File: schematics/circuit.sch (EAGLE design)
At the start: 39 parts, among them IC2 TLC271D, U1 AD5241BRU1M-REEL7AD5241BRZ1M, X1 87758-1816

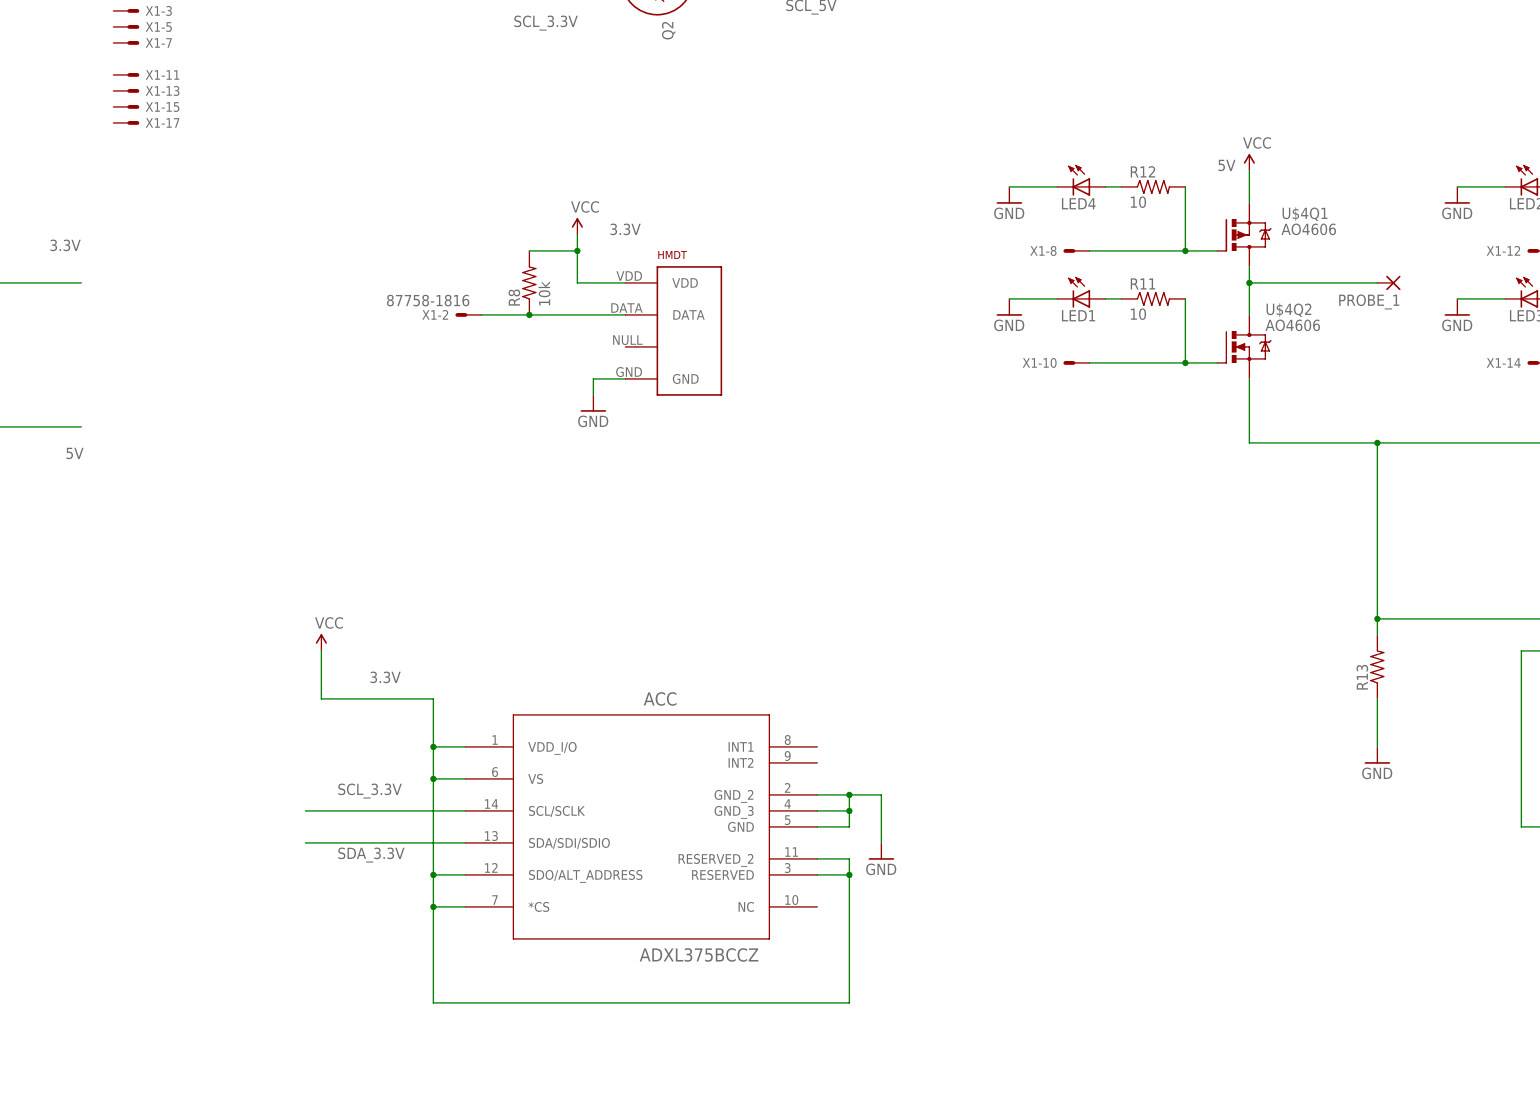
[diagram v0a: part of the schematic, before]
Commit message: почти закончили схему (кроме пережигателей, термисторов, выключателей и флешки) + начала разводить плату
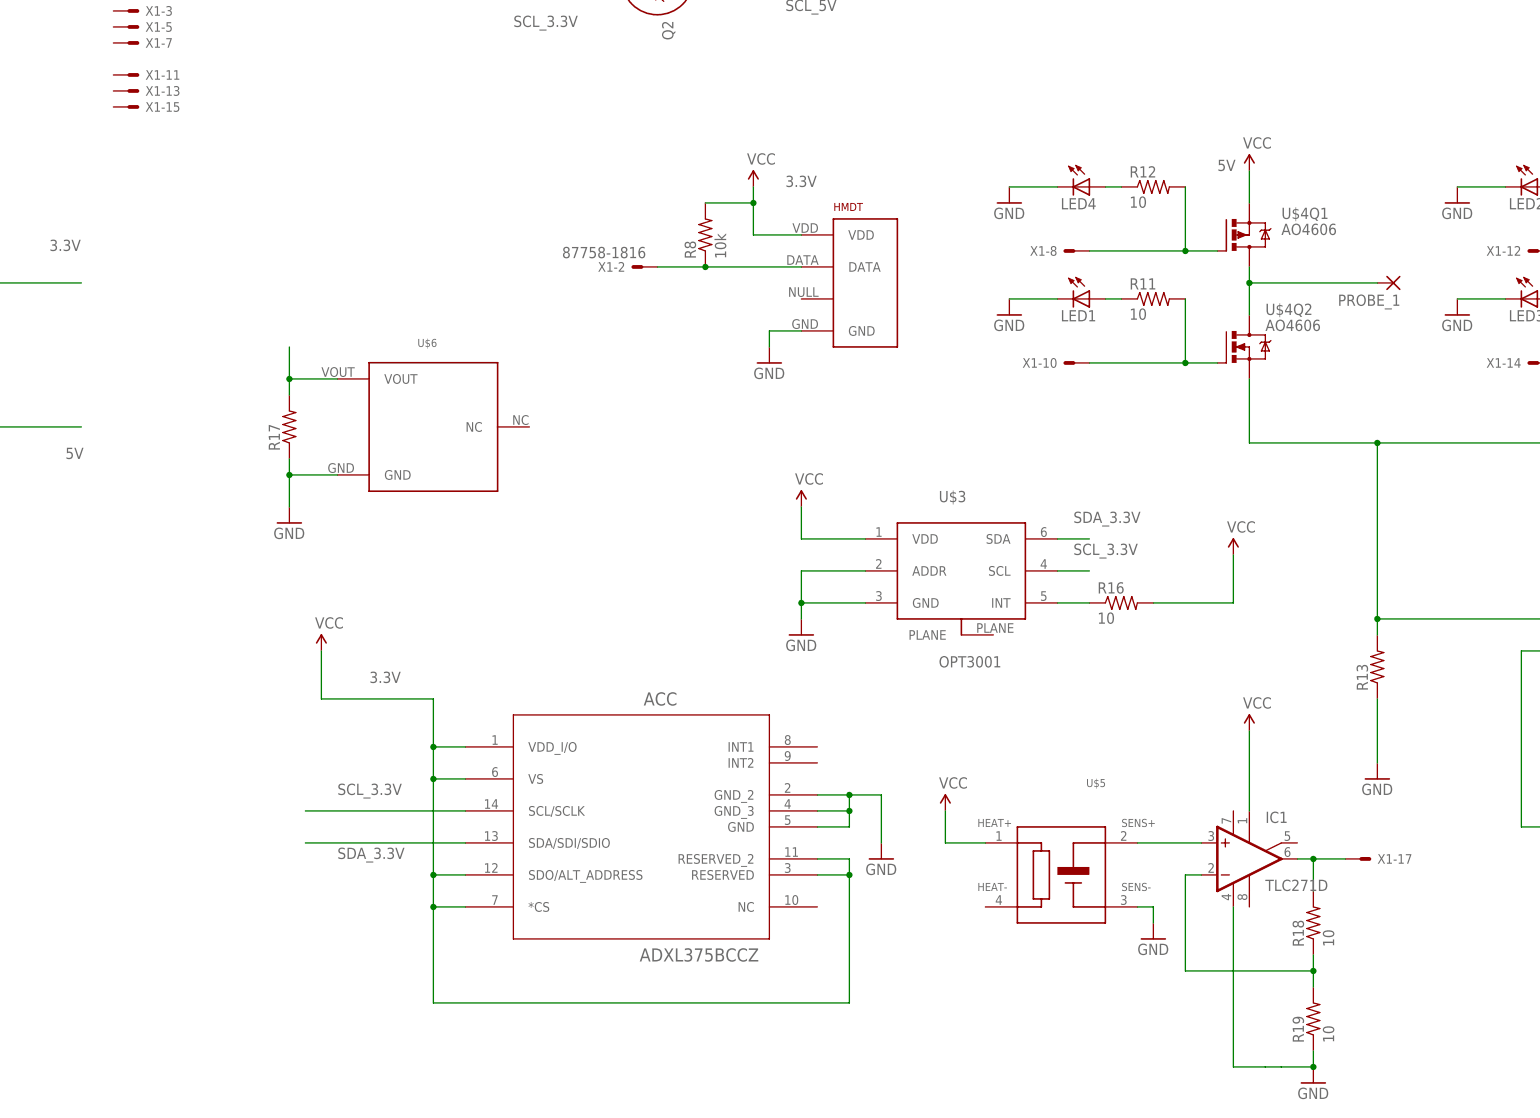
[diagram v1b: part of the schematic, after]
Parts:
- added IC1: TLC271D, linear:TLC271D
- added R16, R18, R19: 10, SparkFun-Resistors:RESISTOR0402
- added R17: (no value), SparkFun-Passives:RESISTOR0402-RES
- added U$3: OPT3001, datchiki:OPT3001
- added U$5: TGS4161, datchiki:TGS4161
- added U$6: O2-A2, datchiki:O2-A2
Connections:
- new net N$19: R16.1, U$3.INT
- new net N$22: IC1.+IN, U$5.SENS+
- new net N$24: IC1.OUT, R18.2, X1-17.S
- net 3.3V: now also R16.2, U$3.VDD
- net 5V: now also IC1.-IN, IC1.ON1, R17.2, R18.1, R19.2, U$5.HEAT+, U$6.VOUT
- net GND: now also IC1.V-, R17.1, R19.1, U$3.ADDR, U$3.GND, U$5.SENS-, U$6.GND
- net SCL_3.3V: now also U$3.SCL
- net SDA_3.3V: now also U$3.SDA
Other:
- moved on the sheet: HMDT, R8, X1-17, X1-2
